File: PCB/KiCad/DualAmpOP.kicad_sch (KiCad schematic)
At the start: 8 parts, among them J1 Conn_01x06_Pin, P1 value, U1 MCP6002

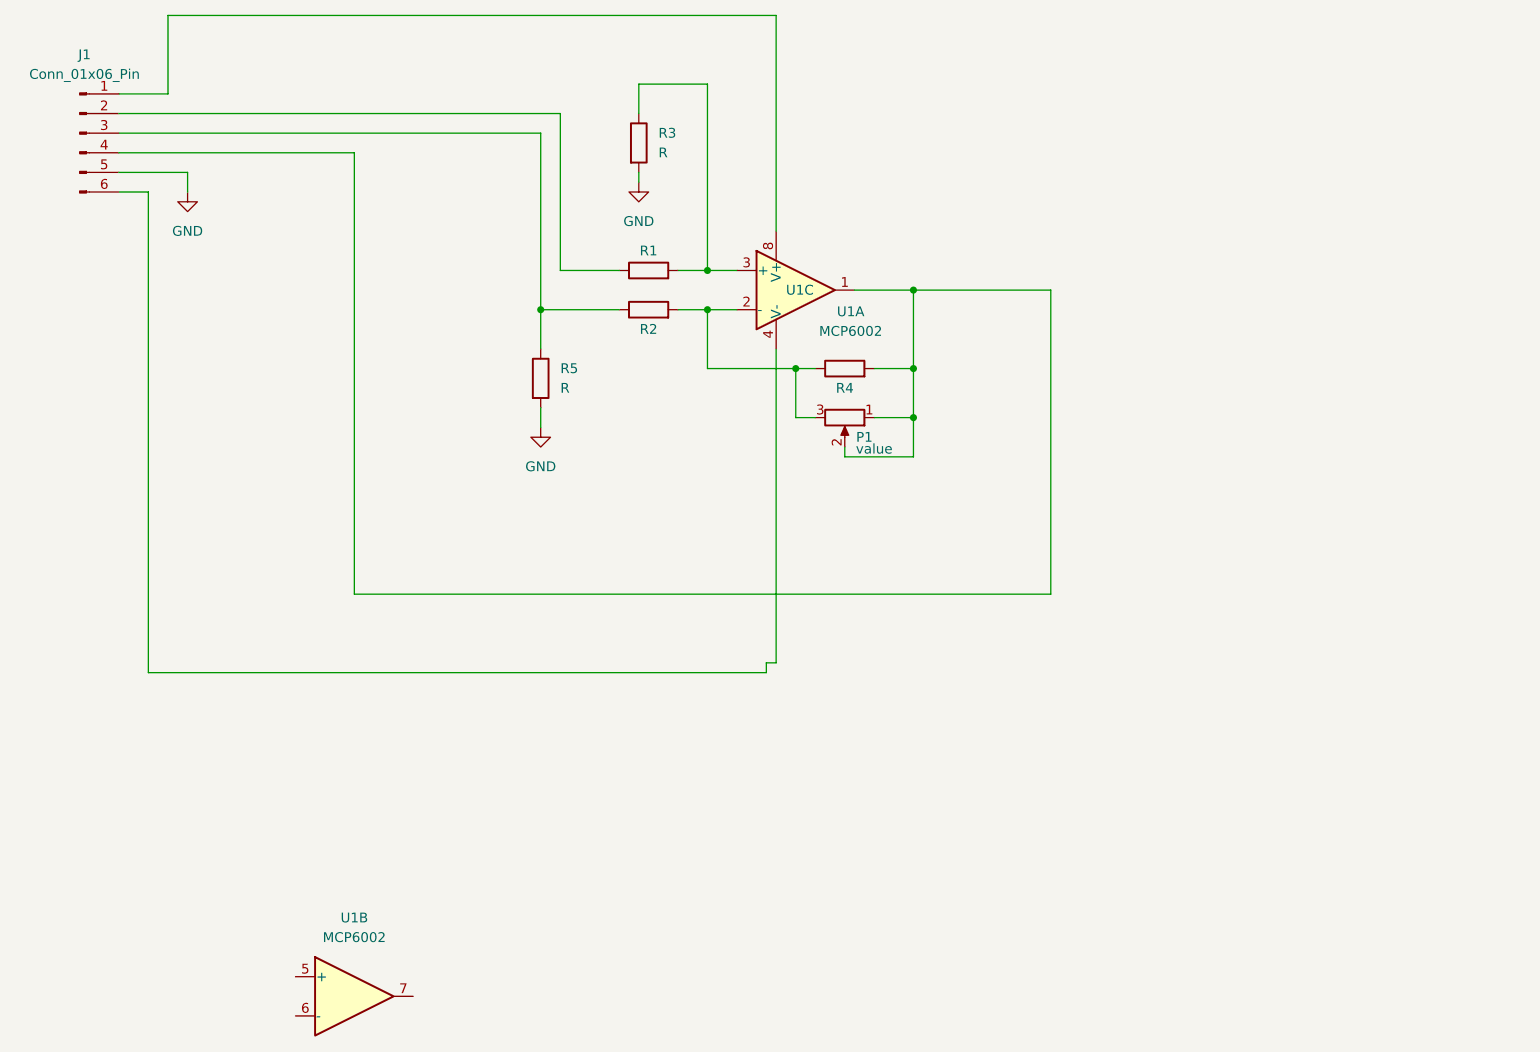
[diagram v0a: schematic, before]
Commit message: Nouvelle version 2 plus pratique
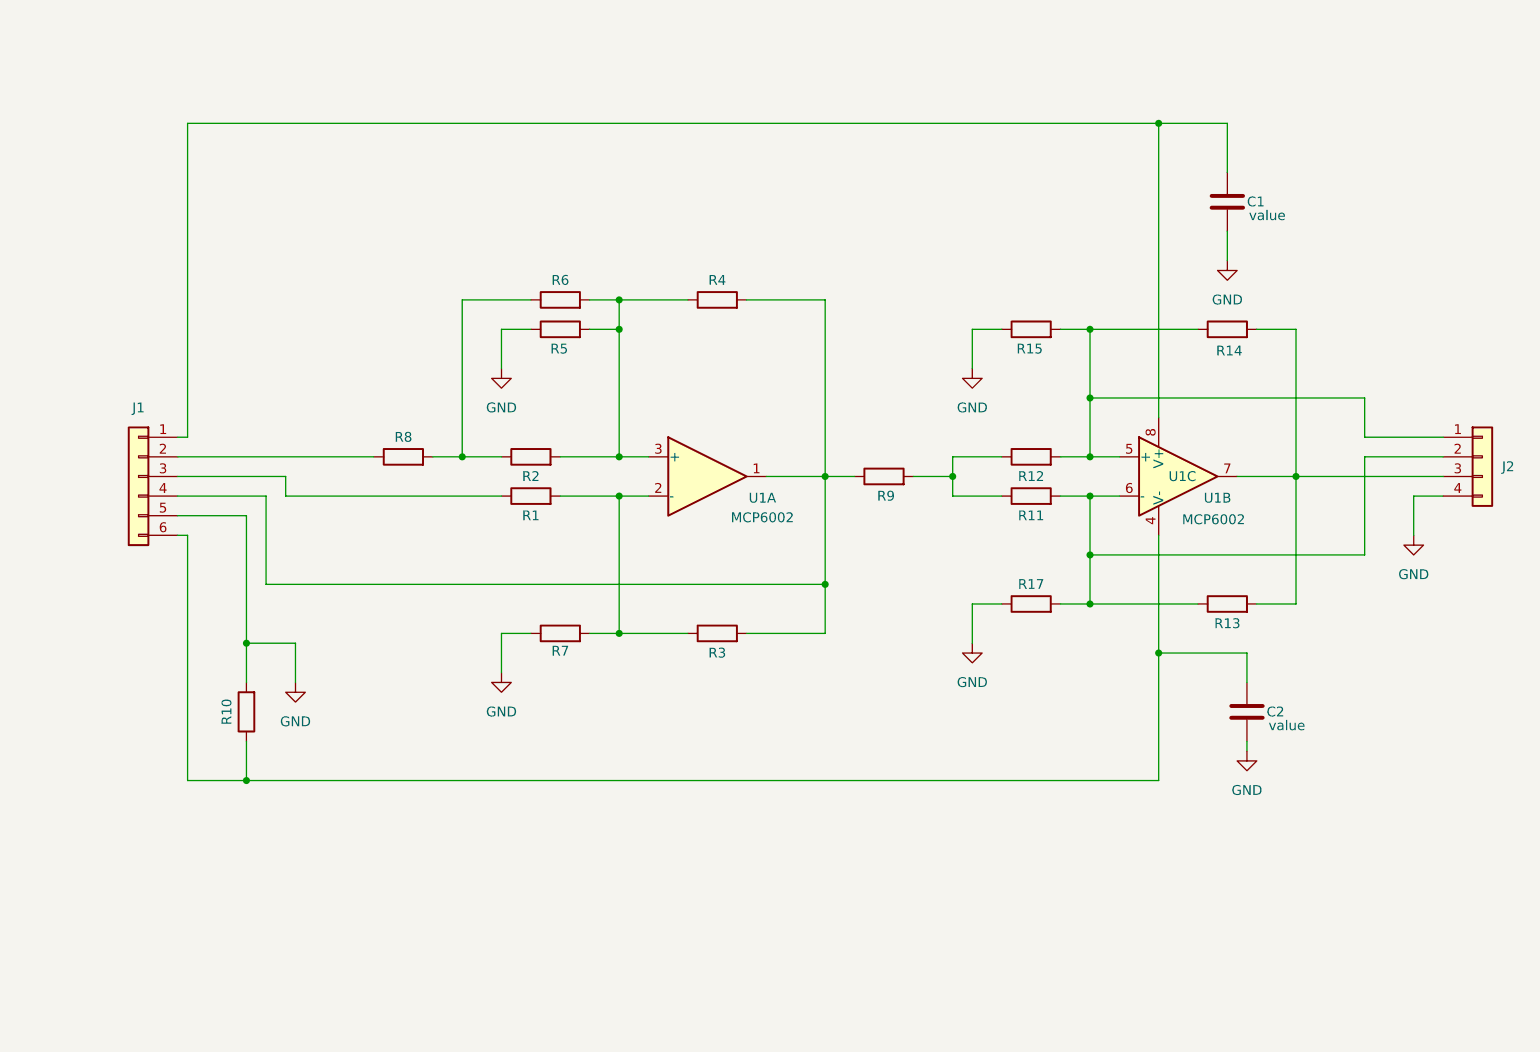
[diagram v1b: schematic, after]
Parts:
- removed J1: Conn_01x06_Pin, symbol Connector:Conn_01x06_Pin
- removed P1: value, 00_Resistor:Potentiometer_Bourns_3296W_Vertical, symbol 00_Resistor:Trimmer_Potentiometer_model
- removed unit 2 of U1
- added C1, C2: value, 00_Capacitor:C_0805_2012Metric_Pad1.18x1.45mm_HandSolder, symbol 00_Capacitor:C_0805
- added J1: (no value), Connector_PinHeader_2.54mm:PinHeader_1x06_P2.54mm_Vertical, symbol 00_Connector:Pin_01x06
- added J2: (no value), Connector_PinHeader_2.54mm:PinHeader_1x04_P2.54mm_Vertical, symbol 00_Connector:Pin_01x04
- added R10, R14, R17, R6, R7, R8, R9: value, Resistor_SMD:R_0805_2012Metric_Pad1.20x1.40mm_HandSolder, symbol 00_Resistor:R_0805
- added R11, R12, R13, R15: R, Resistor_SMD:R_0805_2012Metric_Pad1.20x1.40mm_HandSolder, symbol Device:R
- added unit 2 of U1
- R1: renamed from R2; footprint (none) -> Resistor_SMD:R_0805_2012Metric_Pad1.20x1.40mm_HandSolder
- R2: renamed from R4; footprint (none) -> Resistor_SMD:R_0805_2012Metric_Pad1.20x1.40mm_HandSolder
- R3, R5: footprint (none) -> Resistor_SMD:R_0805_2012Metric_Pad1.20x1.40mm_HandSolder
- R4: renamed from R1; footprint 00_Resistor:R_0805_2012Metric_Pad1.20x1.40mm_HandSolder -> Resistor_SMD:R_0805_2012Metric_Pad1.20x1.40mm_HandSolder
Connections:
- net GND: now also R5.1, C1.2, C2.2, J1.5 (Pin_5), J2.4 (Pin_4), R10.2, R15.1, R17.1, R7.1; no longer R3.2, R5.2
- net at R1.1: now also J1.3 (Pin_3); no longer R5.1
- net at R1.2, U1.2 (-): now also R3.1, R7.2; no longer R2.1
- net at U1.1: now also R3.2, R4.2, J1.4 (Pin_4), R9.1; no longer R2.2
- net at R4.1: now also R2.2, R5.2, U1.3 (+), R6.2
- net at U1.4 (V-): now also C2.1, J1.6 (Pin_6), R10.1
- net at U1.8 (V+): now also C1.1, J1.1 (Pin_1)
- new net: J2.1 (Pin_1), R12.2, R14.1, R15.2, U1.5 (+)
- new net: J2.2 (Pin_2), R11.2, R13.1, R17.2, U1.6 (-)
- new net: J2.3 (Pin_3), R13.2, R14.2, U1.7
- new net: R11.1, R12.1, R9.2
- new net: R2.1, R6.1, R8.2
- new net: J1.2 (Pin_2), R8.1
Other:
- moved on the sheet: R1, R2, R3, R4, R5, U1A, U1C
